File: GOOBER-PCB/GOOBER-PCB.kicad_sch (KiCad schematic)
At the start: 26 parts, among them J1 XT30U_F, J2 Conn_01x22, J3 Conn_01x22, J6 XT30U_F, Q2 PJD15P06A_L2_00001, U1 TPS565208

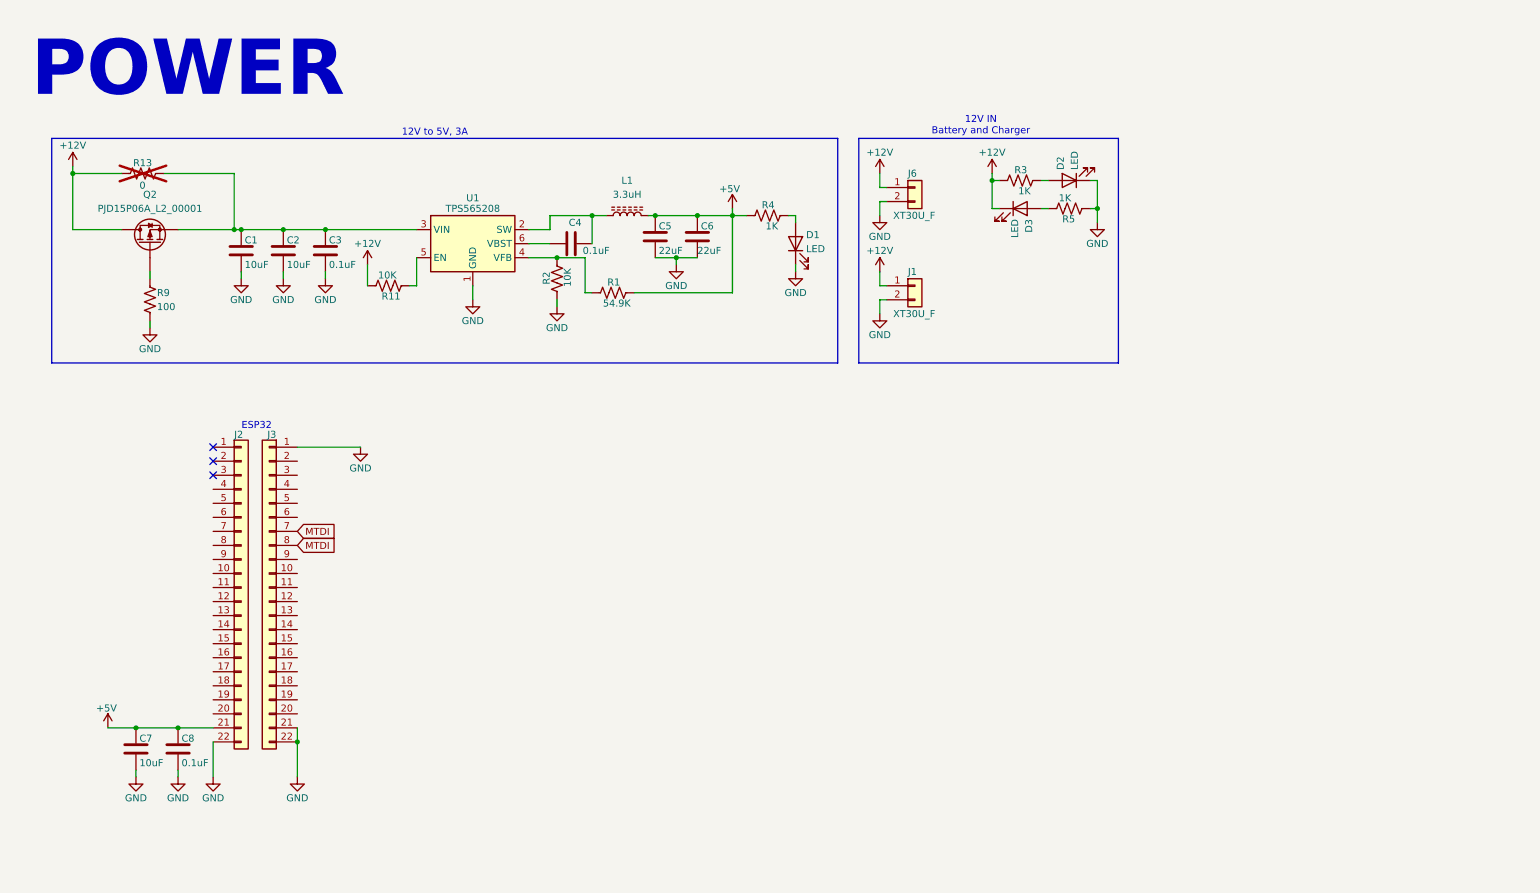
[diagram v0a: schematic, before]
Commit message: did a lot of work for schematic
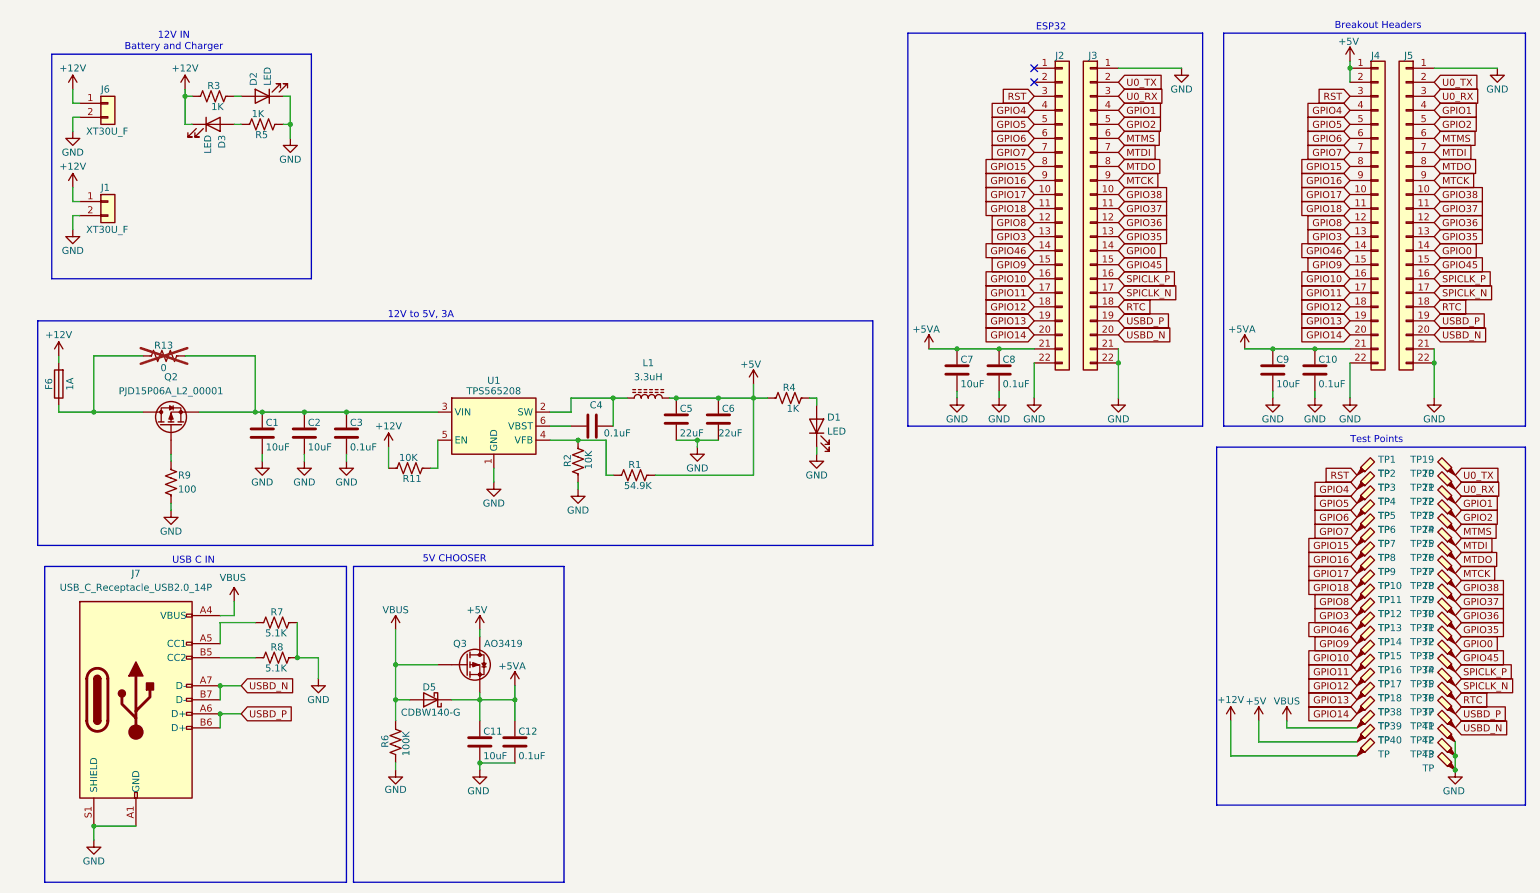
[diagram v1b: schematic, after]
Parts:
- added C10, C12: 0.1uF, Capacitor_SMD:C_0805_2012Metric_Pad1.18x1.45mm_HandSolder, symbol Device:C
- added C11, C9: 10uF, Capacitor_SMD:C_0805_2012Metric_Pad1.18x1.45mm_HandSolder, symbol Device:C
- added D5: CDBW140-G, Diode_SMD:D_SOD-123, symbol Device:D_Schottky
- added F6: 1A, Fuse:Fuseholder_Blade_Mini_Keystone_3568, symbol Device:Fuse
- added J4, J5: Conn_01x22, Connector_PinHeader_2.54mm:PinHeader_1x22_P2.54mm_Vertical, symbol Connector_Generic:Conn_01x22
- added J7: USB_C_Receptacle_USB2.0_14P, Connector_USB:USB_C_Receptacle_GCT_USB4115-03-C, symbol Connector:USB_C_Receptacle_USB2.0_14P
- added Q3: AO3419, Package_TO_SOT_SMD:SOT-23, symbol Device:Q_PMOS
- added R6: 100K, Resistor_SMD:R_0805_2012Metric_Pad1.20x1.40mm_HandSolder, symbol Device:R_US
- added R7, R8: 5.1K, Resistor_SMD:R_0805_2012Metric_Pad1.20x1.40mm_HandSolder, symbol Device:R_US
- added TP1, TP10, TP11, TP12, TP13, TP14, TP15, TP16, TP17, TP18, TP19, TP2, TP20, TP21, TP22, TP23, TP24, TP25, TP26, TP27, TP28, TP29, TP3, TP30, TP31, TP32, TP33, TP34, TP35, TP36, TP37, TP38, TP39, TP4, TP40, TP41, TP42, TP43, TP5, TP6, TP7, TP8, TP9: TP, TestPoint:TestPoint_Keystone_5000-5004_Miniature, symbol Connector:TestPoint_Probe
- D1, D2, D3: footprint Diode_SMD:D_0805_2012Metric_Pad1.15x1.40mm_HandSolder -> LED_SMD:LED_0805_2012Metric
- J2, J3: footprint (none) -> Connector_PinHeader_2.54mm:PinHeader_1x22_P2.54mm_Vertical
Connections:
- net +12V: now also F6.2, TP40.1; no longer Q2.D, R13.2
- net +5V: now also J4.1 (Pin_1), J4.2 (Pin_2), Q3.D, TP39.1; no longer C7.1, C8.1, J2.21 (Pin_21)
- net GND: now also C10.2, C11.2, C12.2, C9.2, J4.22 (Pin_22), J5.1 (Pin_1), J5.21 (Pin_21), J5.22 (Pin_22), J7.A1 (GND), J7.A12 (GND), J7.B1 (GND), J7.B12 (GND), J7.S1 (SHIELD), R6.1, R7.2, R8.2, TP41.1, TP42.1, TP43.1
- net MTDI: now also J5.7 (Pin_7), TP24.1; no longer J3.8 (Pin_8)
- net GPIO17: now reaches J2.10 (Pin_10)
- net GPIO17: now also J4.10 (Pin_10), TP8.1
- net GPIO18: now reaches J2.11 (Pin_11)
- net GPIO18: now also J4.11 (Pin_11), TP9.1
- net GPIO8: now reaches J2.12 (Pin_12)
- net GPIO8: now also J4.12 (Pin_12), TP10.1
- net GPIO3: now reaches J2.13 (Pin_13)
- net GPIO3: now also J4.13 (Pin_13), TP11.1
- net GPIO46: now reaches J2.14 (Pin_14)
- net GPIO46: now also J4.14 (Pin_14), TP12.1
- net GPIO9: now reaches J2.15 (Pin_15)
- net GPIO9: now also J4.15 (Pin_15), TP13.1
- net GPIO10: now reaches J2.16 (Pin_16)
- net GPIO10: now also J4.16 (Pin_16), TP14.1
- net GPIO11: now reaches J2.17 (Pin_17)
- net GPIO11: now also J4.17 (Pin_17), TP15.1
- net GPIO12: now reaches J2.18 (Pin_18)
- net GPIO12: now also J4.18 (Pin_18), TP16.1
- net GPIO13: now reaches J2.19 (Pin_19)
- net GPIO13: now also J4.19 (Pin_19), TP17.1
- net GPIO14: now reaches J2.20 (Pin_20)
- net GPIO14: now also J4.20 (Pin_20), TP18.1
- net RST: now reaches J2.3 (Pin_3)
- net RST: now also J4.3 (Pin_3), TP1.1
- net GPIO4: now reaches J2.4 (Pin_4)
- net GPIO4: now also J4.4 (Pin_4), TP2.1
- net GPIO5: now reaches J2.5 (Pin_5)
- net GPIO5: now also J4.5 (Pin_5), TP3.1
- net GPIO6: now reaches J2.6 (Pin_6)
- net GPIO6: now also J4.6 (Pin_6), TP4.1
- net GPIO7: now reaches J2.7 (Pin_7)
- net GPIO7: now also J4.7 (Pin_7), TP5.1
- net GPIO15: now reaches J2.8 (Pin_8)
- net GPIO15: now also J4.8 (Pin_8), TP6.1
- net GPIO16: now reaches J2.9 (Pin_9)
- net GPIO16: now also J4.9 (Pin_9), TP7.1
- net GPIO38: now reaches J3.10 (Pin_10)
- net GPIO38: now also J5.10 (Pin_10), TP27.1
- net GPIO37: now reaches J3.11 (Pin_11)
- net GPIO37: now also J5.11 (Pin_11), TP28.1
- net GPIO36: now reaches J3.12 (Pin_12)
- net GPIO36: now also J5.12 (Pin_12), TP29.1
- net GPIO35: now reaches J3.13 (Pin_13)
- net GPIO35: now also J5.13 (Pin_13), TP30.1
- net GPIO0: now reaches J3.14 (Pin_14)
- net GPIO0: now also J5.14 (Pin_14), TP31.1
- net GPIO45: now reaches J3.15 (Pin_15)
- net GPIO45: now also J5.15 (Pin_15), TP32.1
- net SPICLK_P: now reaches J3.16 (Pin_16)
- net SPICLK_P: now also J5.16 (Pin_16), TP33.1
- net SPICLK_N: now reaches J3.17 (Pin_17)
- net SPICLK_N: now also J5.17 (Pin_17), TP34.1
- net RTC: now reaches J3.18 (Pin_18)
- net RTC: now also J5.18 (Pin_18), TP35.1
- net USBD_P: now reaches J3.19 (Pin_19)
- net USBD_P: now also J5.19 (Pin_19), J7.A6 (D+), J7.B6 (D+), TP36.1
- net U0_TX: now reaches J3.2 (Pin_2)
- net U0_TX: now also J5.2 (Pin_2), TP19.1
- net USBD_N: now reaches J3.20 (Pin_20)
- net USBD_N: now also J5.20 (Pin_20), J7.A7 (D-), J7.B7 (D-), TP37.1
- net U0_RX: now reaches J3.3 (Pin_3)
- net U0_RX: now also J5.3 (Pin_3), TP20.1
- net GPIO1: now reaches J3.4 (Pin_4)
- net GPIO1: now also J5.4 (Pin_4), TP21.1
- net GPIO2: now reaches J3.5 (Pin_5)
- net GPIO2: now also J5.5 (Pin_5), TP22.1
- net MTMS: now reaches J3.6 (Pin_6)
- net MTMS: now also J5.6 (Pin_6), TP23.1
- net MTCK: now reaches J3.9 (Pin_9)
- net MTCK: now also J5.9 (Pin_9), TP26.1
- new net: F6.1, Q2.D, R13.2
- new net: J7.A5 (CC1), R7.1
- new net: J7.B5 (CC2), R8.1
- new net +5VA: C10.1, C11.1, C12.1, C7.1, C8.1, C9.1, D5.1 (K), J2.21 (Pin_21), J4.21 (Pin_21), Q3.S
- new net MTDO: J3.8 (Pin_8), J5.8 (Pin_8), TP25.1
- new net VBUS: D5.2 (A), J7.A4 (VBUS), J7.A9 (VBUS), J7.B4 (VBUS), J7.B9 (VBUS), Q3.G, R6.2, TP38.1
- no-connect marks 3 -> 2
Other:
- note added: "5V CHOOSER"
- note added: "Breakout Headers"
- note added: "Test Points"
- note added: "USB C IN"
- note removed: "POWER"
- moved on the sheet: C1, C2, C3, C4, C5, C6, C7, C8, D1, D2, D3, J1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
